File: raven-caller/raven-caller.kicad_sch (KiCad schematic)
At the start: 13 parts, among them J1 I2C LCD, Q1 BSS138, SW1 RotaryEncoder_Switch, U1 SeeeduinoXIAO, U2 RFM95W-915S2, U3 24LC256, U4 PCF8574AP

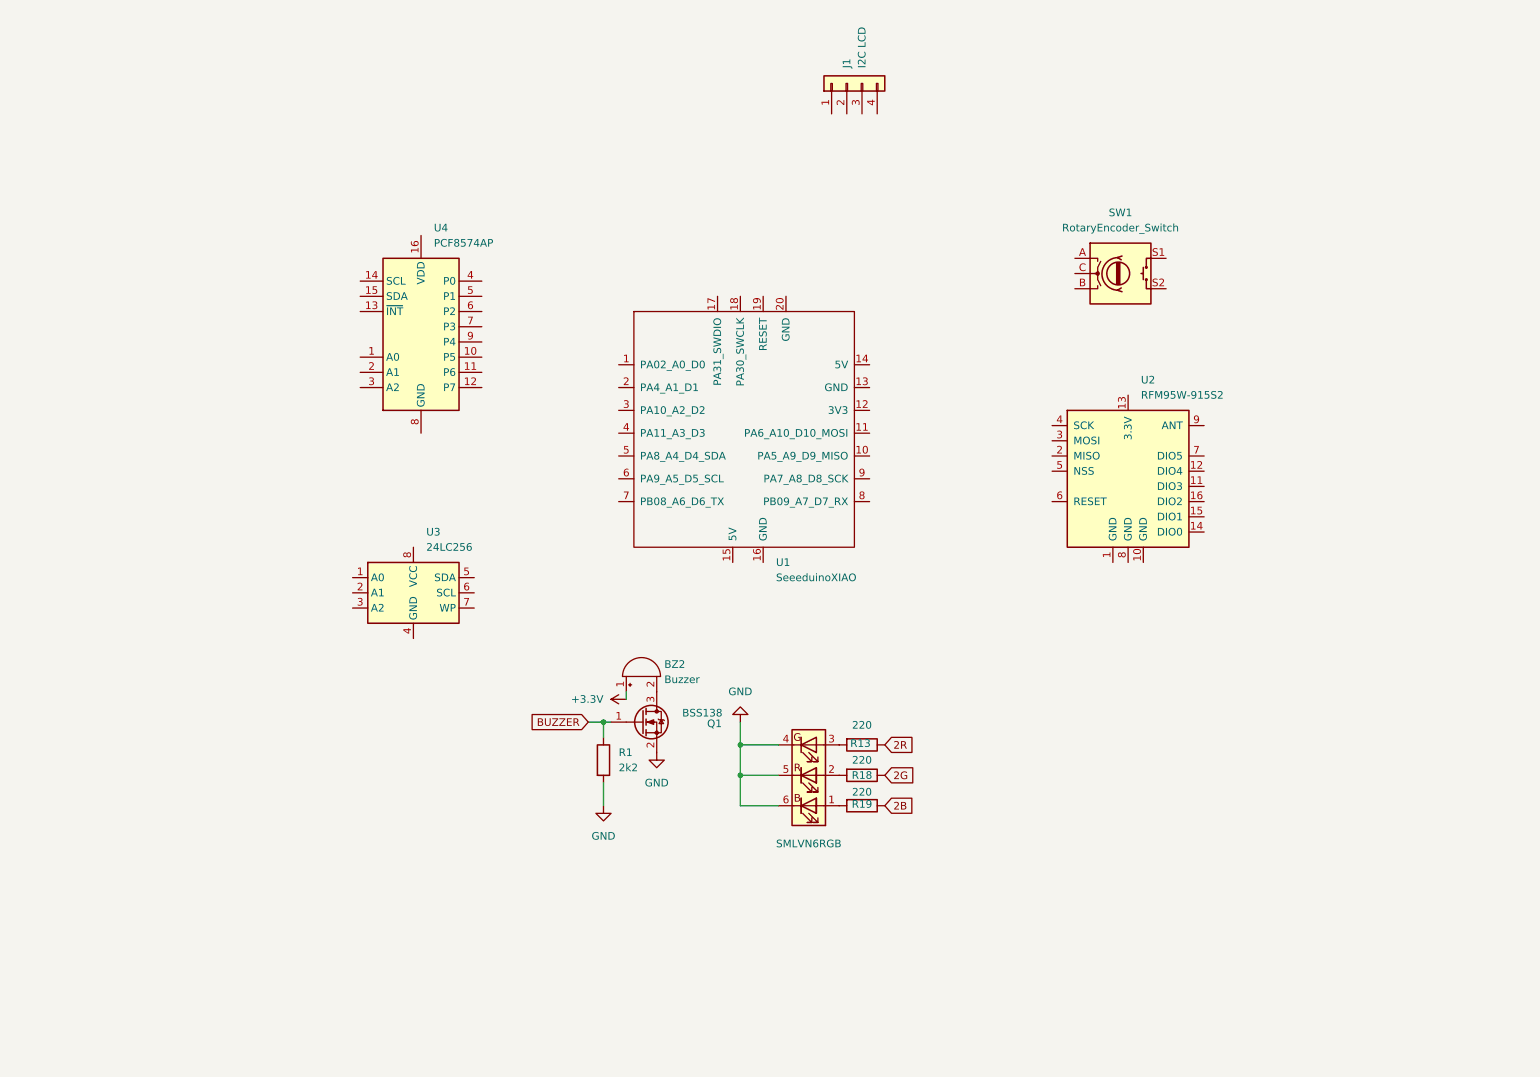
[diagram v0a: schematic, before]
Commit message: schematic v1 done
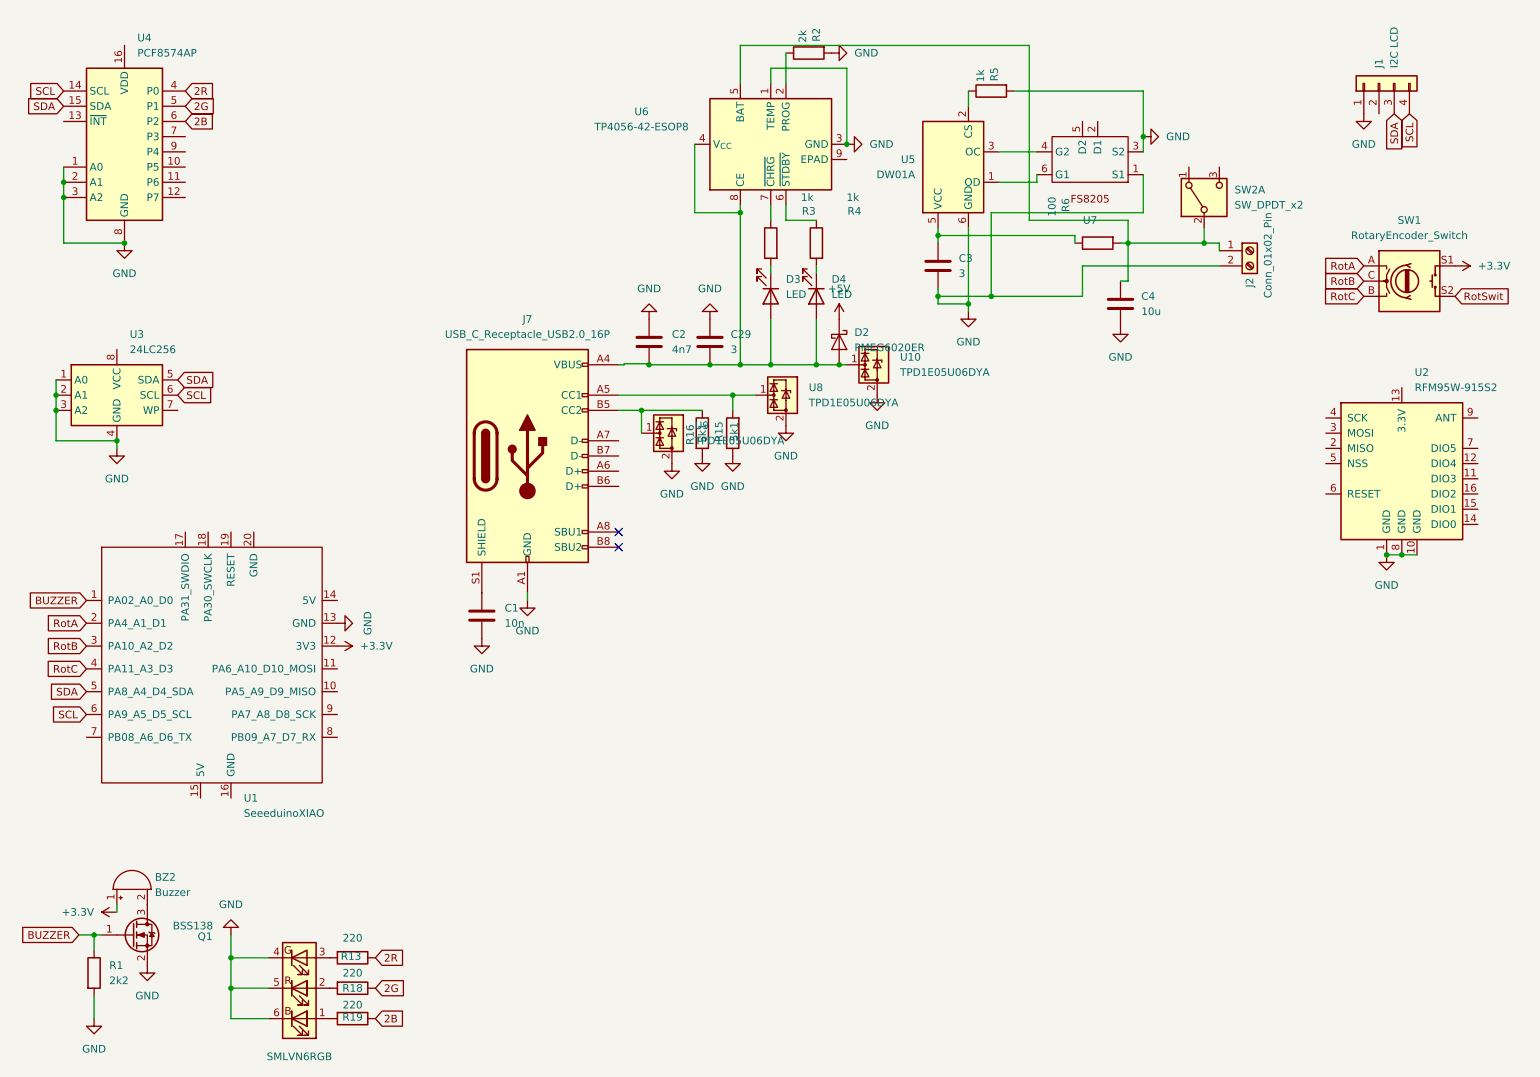
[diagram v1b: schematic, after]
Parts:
- added C1: 10n, Capacitor_SMD:C_0603_1608Metric, symbol Device:C
- added C2: 4n7, Capacitor_SMD:C_0603_1608Metric, symbol Device:C
- added C29, C3: 3, Capacitor_SMD:C_0603_1608Metric, symbol Device:C
- added C4: 10u, Capacitor_SMD:C_0603_1608Metric, symbol Device:C
- added D2: PMEG6020ER, Diode_SMD:Nexperia_CFP3_SOD-123W, symbol Diode:PMEG6020ER
- added D3, D4: LED, LED_SMD:LED_0603_1608Metric, symbol Device:LED
- added J2: Conn_01x02_Pin, Connector_JST:JST_PH_B2B-PH-K_1x02_P2.00mm_Vertical, symbol Connector:Screw_Terminal_01x02
- added J7: USB_C_Receptacle_USB2.0_16P, Connector_USB:USB_C_Receptacle_GCT_USB4105-xx-A_16P_TopMnt_Horizontal, symbol Connector:USB_C_Receptacle_USB2.0_16P
- added R15, R16: 5k1, Resistor_SMD:R_0603_1608Metric, symbol Device:R
- added R2: 2k, Resistor_SMD:R_0603_1608Metric, symbol Device:R
- added R3, R4, R5: 1k, Resistor_SMD:R_0603_1608Metric, symbol Device:R
- added R6: 100, Resistor_SMD:R_0603_1608Metric, symbol Device:R
- added SW2: SW_DPDT_x2, symbol Switch:SW_DPDT_x2
- added U10, U8, U9: TPD1E05U06DYA, Diode_SMD:D_SOD-523, symbol Power_Protection:TPD1E05U06DYA
- added U5: DW01A, Package_TO_SOT_SMD:SOT-23-6, symbol Battery_Management:DW01A
- added U6: TP4056-42-ESOP8, Package_SO:SOIC-8-1EP_3.9x4.9mm_P1.27mm_EP2.41x3.3mm_ThermalVias, symbol Battery_Management:TP4056-42-ESOP8
- added U7: ~, Package_TO_SOT_SMD:SOT-23-6, symbol FS8205:FS8205
- J1: footprint (none) -> Connector_PinHeader_2.54mm:PinHeader_1x04_P2.54mm_Horizontal
- SW1: footprint (none) -> Rotary_Encoder:RotaryEncoder_Alps_EC11E-Switch_Vertical_H20mm
- U1: footprint (none) -> Xiao Seeed SAMD21:XiaoSeeed
- U3: footprint (none) -> Package_SO:SOIC-8_3.9x4.9mm_P1.27mm
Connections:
- net +3.3V: now also SW1.S1, U1.12 (3V3)
- net 2B: now also U4.6 (P2)
- net 2G: now also U4.5 (P1)
- net 2R: now also U4.4 (P0)
- net BUZZER: now also U1.1 (PA02_A0_D0)
- net GND: now also J1.1 (Pin_1), U1.13 (GND), U2.1 (GND), U2.10 (GND), U2.8 (GND), U3.1 (A0), U3.2 (A1), U3.3 (A2), U3.4 (GND), U4.1 (A0), U4.2 (A1), U4.3 (A2), U4.8 (GND), C1.2, C2.1, C29.1, C3.2, C4.2, J2.2 (Pin_2), J7.A1 (GND), J7.A12 (GND), J7.B1 (GND), J7.B12 (GND), R15.1, R16.2, R2.2, R5.2, U10.2 (GND), U5.6 (GND), U6.1 (TEMP), U6.3 (GND), U7.1 (S1), U7.3 (S2), U8.2 (GND), U9.2 (GND)
- net SDA: now reaches U3.5 (SDA)
- net SDA: now also J1.3 (Pin_3), U1.5 (PA8_A4_D4_SDA), U4.15 (SDA)
- net SCL: now reaches U3.6 (SCL)
- net SCL: now also J1.4 (Pin_4), U1.6 (PA9_A5_D5_SCL), U4.14 (SCL)
- net RotA: now reaches SW1.A
- net RotA: now also U1.2 (PA4_A1_D1)
- net RotC: now reaches SW1.B
- net RotC: now also U1.4 (PA11_A3_D3)
- net RotB: now reaches SW1.C
- net RotB: now also U1.3 (PA10_A2_D2)
- net RotSwit: now reaches SW1.S2
- new net: U5.3 (OC), U7.4 (G2)
- new net: U5.1 (OD), U7.6 (G1)
- new net: C2.2, C29.2, D2.2 (A), D3.2 (A), D4.2 (A), J7.A4 (VBUS), J7.A9 (VBUS), J7.B4 (VBUS), J7.B9 (VBUS), U10.1 (I/O), U6.4 (V_{CC}), U6.8 (CE)
- new net: C3.1, R6.1, U5.5 (VCC)
- new net: C4.1, J2.1 (Pin_1), R6.2, SW2.2 (B), U6.5 (BAT)
- new net: J7.A5 (CC1), R15.2, U8.1 (I/O)
- new net: D3.1 (K), R3.2
- new net: R3.1, U6.7 (~{CHRG})
- new net: R5.1, U5.2 (CS)
- new net: D4.1 (K), R4.2
- new net: R4.1, U6.6 (~{STDBY})
- new net: J7.B5 (CC2), R16.1, U9.1 (I/O)
- new net: C1.1, J7.S1 (SHIELD)
- new net: R2.1, U6.2 (PROG)
- new net +5V: D2.1 (K)
- no-connect marks 0 -> 2
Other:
- moved on the sheet: BZ2, J1, Q1, R1, R13, R18, R19, SW1, U1, U2, U3, U4
